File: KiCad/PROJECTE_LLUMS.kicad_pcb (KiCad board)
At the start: 2 copper layers, 116.3 x 86.1 mm, 82 parts, among them J1 CONNECTOR_MOTOR, J10 Conn_01x02_Pin, J2 DE9_Pins_MountingHoles, J3 Conn_01x05, J4 Conn_01x02_Pin, J5 DE9_Pins_MountingHoles, J6 Conn_01x02_Pin, J7 Conn_01x02_Pin, J8 Conn_01x02_Pin, J9 Conn_01x02_Pin, K1 Fujitsu_FTR-LYAA005x, Q2 IRLZ44N, Q3 IRLZ44N, Q4 IRLZ44N, Q5 IRLZ44N, Q6 IRLZ44N, Q7 IRLZ44N, SW1 SW_Push, SW2 SW_Push, SW3 SW_Push, SW4 SW_Push, SW5 SW_Push, SW6 SW_Push, U1 BH1750FVI-TR, U4 MCP2551-I-SN, U5 LM2596S-5, U6 LM1117MP-3.3, U7 PIC24HJ128GP502, Y1 8MHz

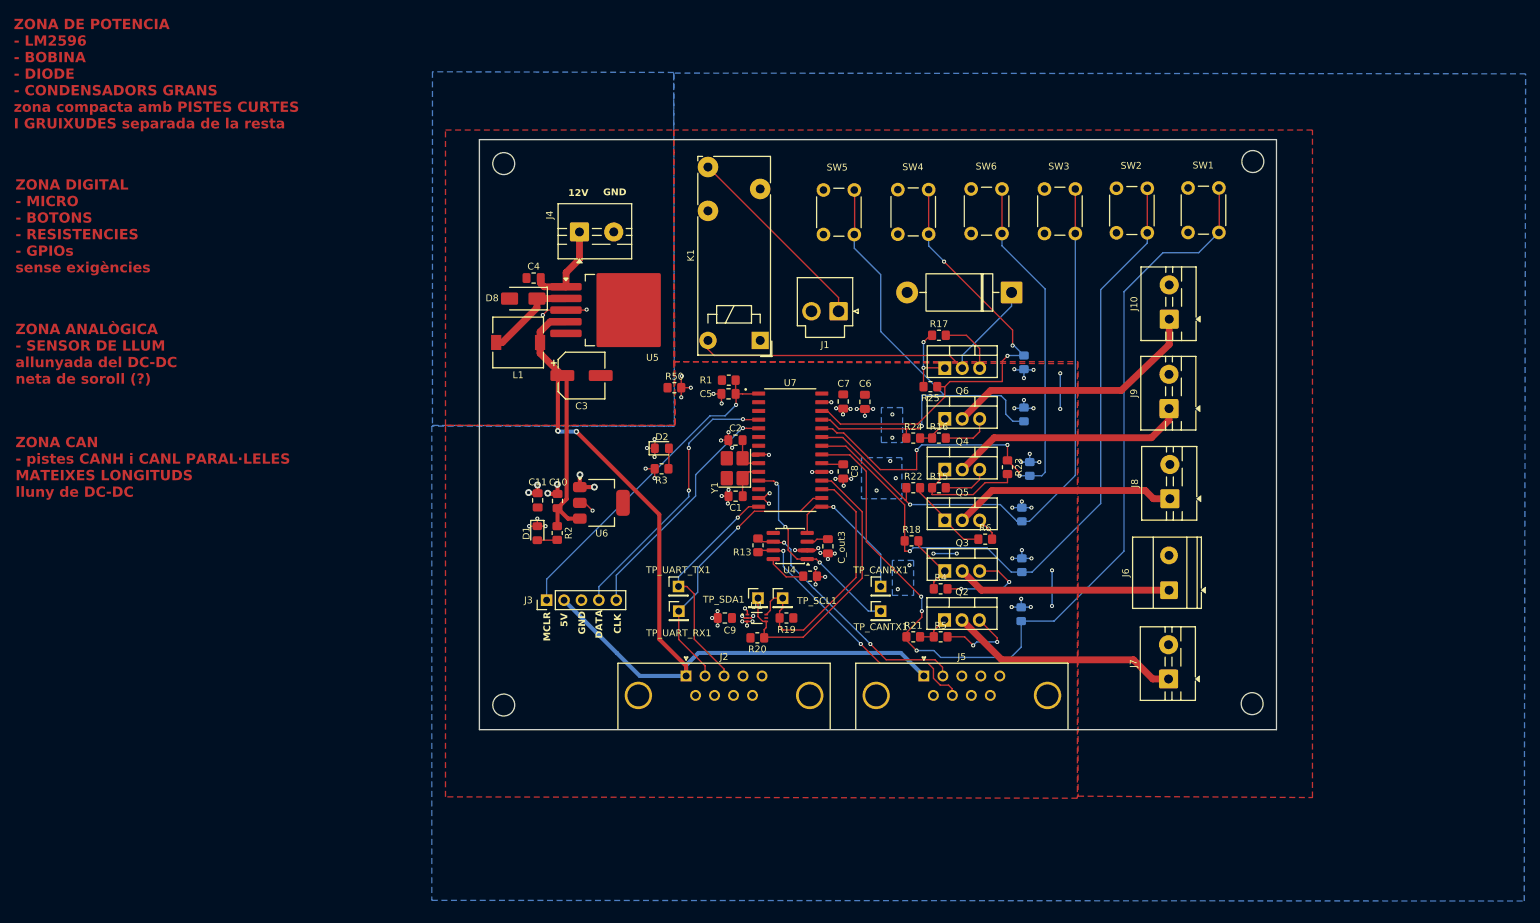
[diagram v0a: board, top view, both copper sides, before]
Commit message: errors finals
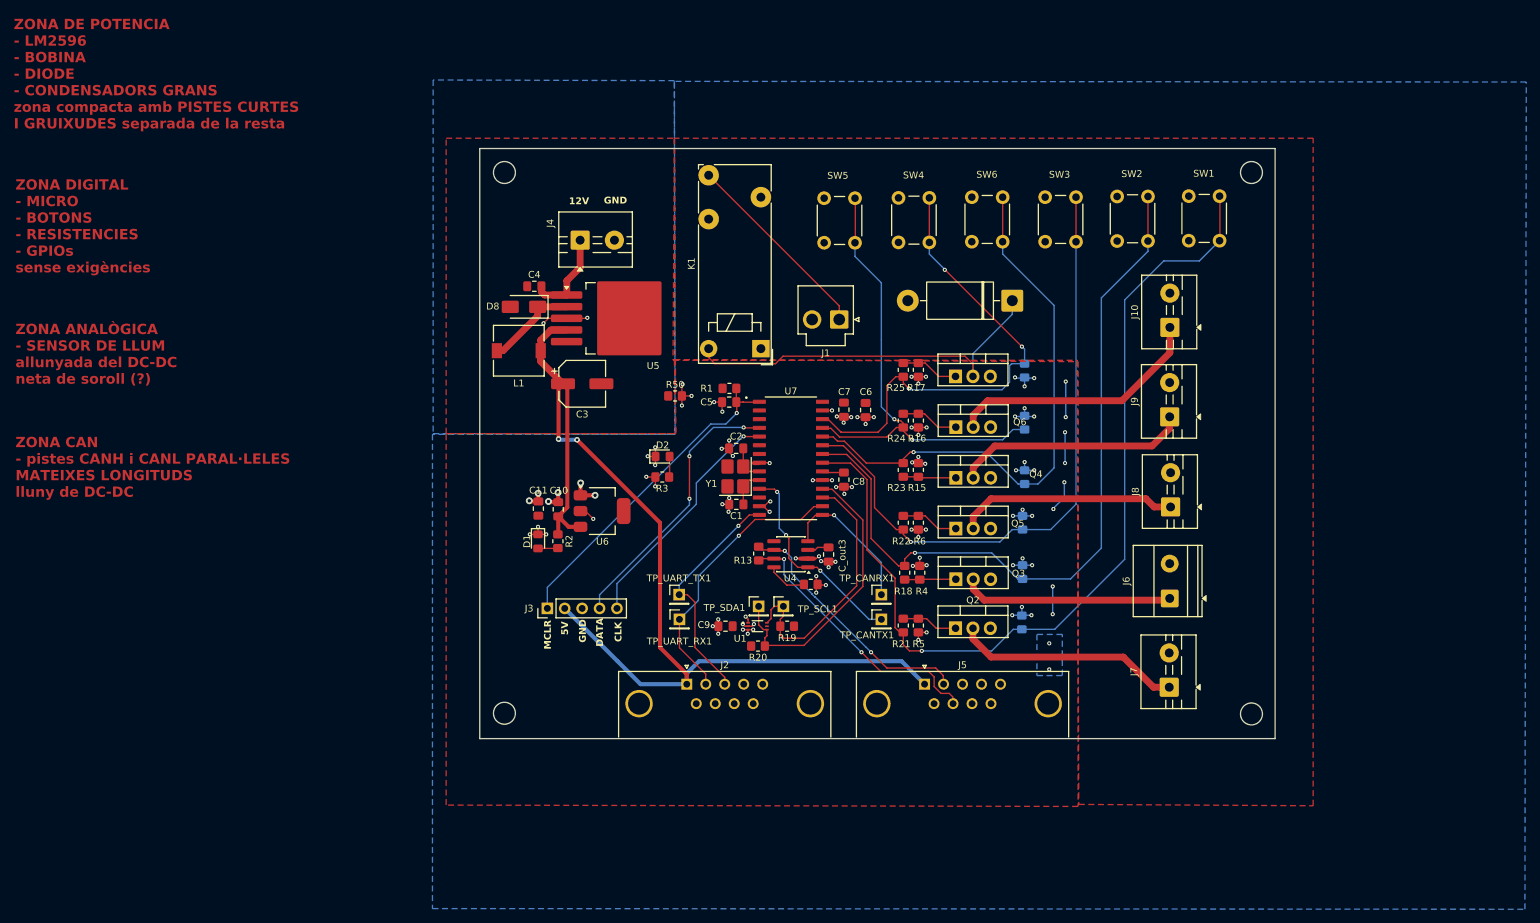
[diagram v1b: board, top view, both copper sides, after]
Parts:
- moved R23 15.2 mm to (148.3, 82.9)
- moved R6 10.0 mm to (150.5, 90.6), turned to -90 degrees
- moved R17 5.87 mm to (150.5, 68.3), turned to -90 degrees
- moved R22 5.30 mm to (148.3, 90.6), turned to 90 degrees
- moved R18 4.76 mm to (148.5, 97.9), turned to -90 degrees
- moved R25 4.65 mm to (148.3, 68.3), turned to 90 degrees
- moved R15 3.97 mm to (150.5, 82.9), turned to 90 degrees
- moved R16 3.94 mm to (150.5, 75.7), turned to -90 degrees
- moved R4 3.85 mm to (150.7, 97.9), turned to 90 degrees
- moved R5 3.64 mm to (150.5, 105.6), turned to -90 degrees
- moved R24 2.93 mm to (148.3, 75.7), turned to 90 degrees
- moved R21 2.20 mm to (148.3, 105.6), turned to 90 degrees
- moved Q2 2.00 mm to (155.9, 106.0)
- moved Q4 2.00 mm to (156.0, 84.0)
- moved Q5 2.00 mm to (156.0, 91.5)
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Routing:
- net GND: track 119.2 -> 84.4 mm, vias 56 -> 69
- net Net-(Q4-G): track 18.0 -> 7.72 mm
- net +3V3: track 43.7 -> 51.4 mm, vias 35 -> 34
- net ENCREUAMENT: track 105.7 -> 111.5 mm
- net CARRETERA: track 139.7 -> 134.1 mm, vias 3 -> 1
- net INTERM. DRT: track 74.3 -> 69.4 mm, vias 1 -> 2
- net DIURNA: track 88.7 -> 93.0 mm
- net INTERM. ESQ: track 85.9 -> 82.0 mm, vias 3 -> 1
- net Net-(Q5-G): track 12.4 -> 8.43 mm
- net Net-(Q2-G): track 4.70 -> 8.20 mm
- net (no net): track 3.50 -> 0.00 mm, vias 2 -> 0
- net Net-(Q6-G): track 5.15 -> 8.47 mm
- net NETEJA-FARS: track 68.5 -> 71.5 mm
- net /llums/RELÉ: track 53.6 -> 56.4 mm
- net Net-(Q7-G): track 10.9 -> 8.43 mm, vias 2 -> 0
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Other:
- board size 116.3 x 86.1 mm -> 116.1 x 86.1 mm
